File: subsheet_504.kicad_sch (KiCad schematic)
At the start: 36 parts, among them J502 Phono LEFT, J503 Phono RIGHT, U504 LF347N_mu, U508 LMC1992CCN_PHY

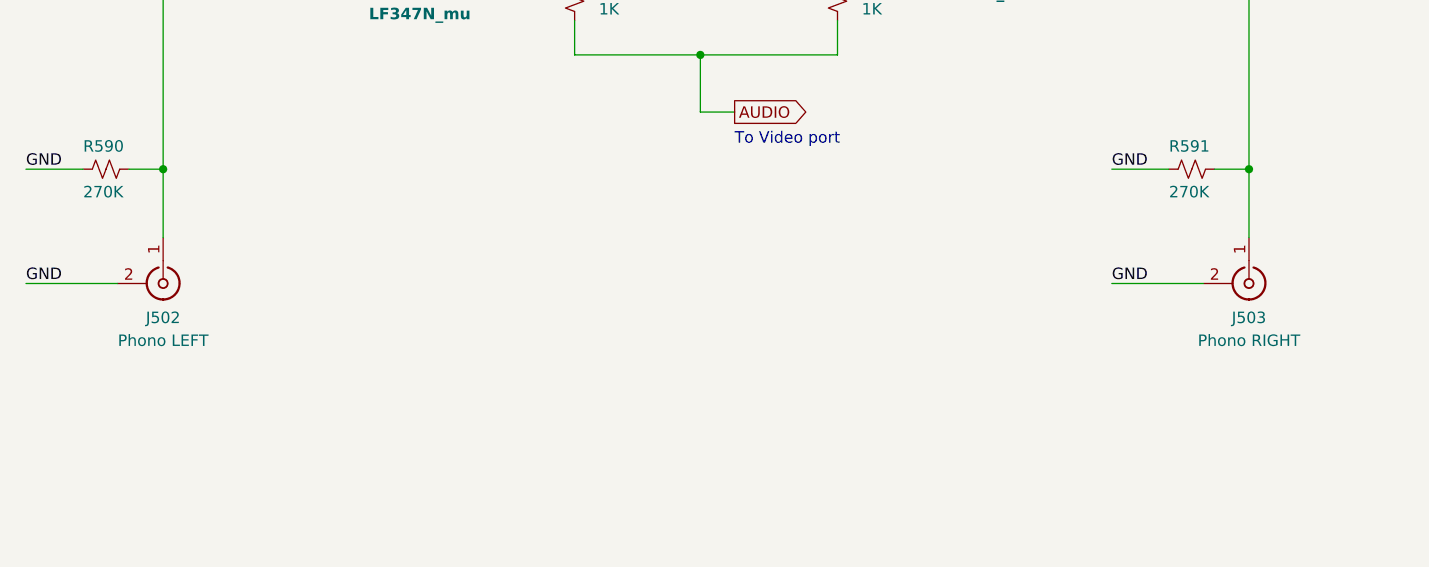
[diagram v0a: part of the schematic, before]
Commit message: pcb session 2023-01-21T22:41:51+01:00
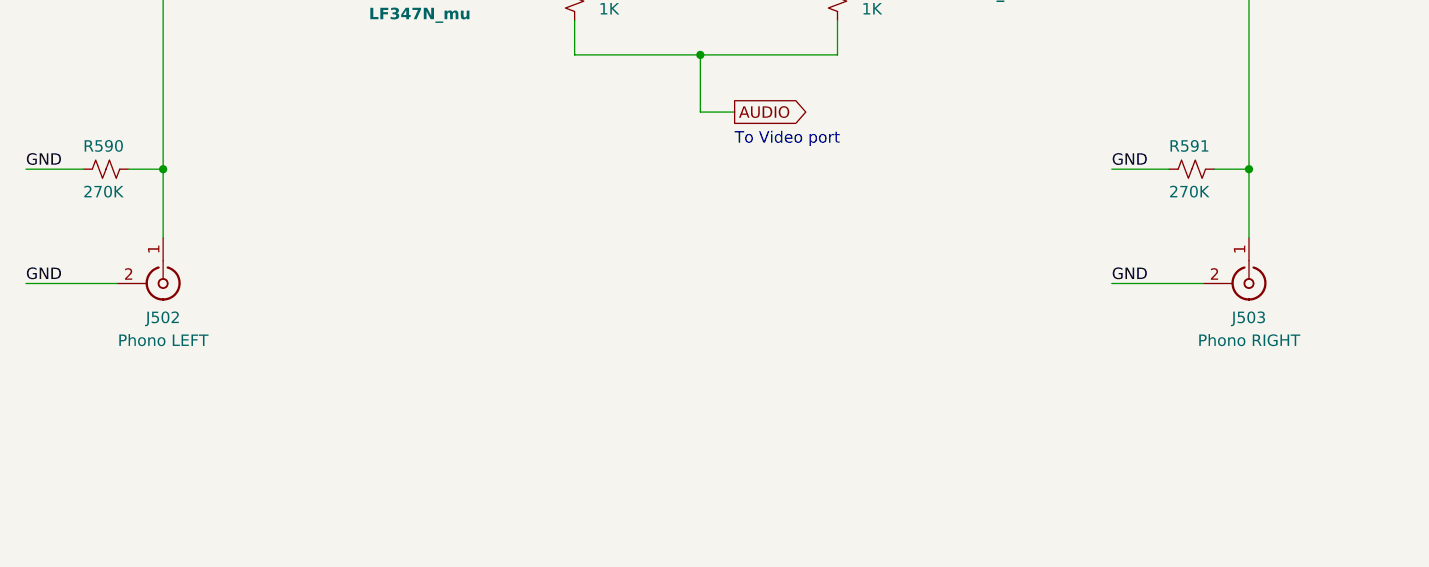
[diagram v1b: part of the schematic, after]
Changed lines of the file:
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@@
     (pin "9")
   )
-  (symbol (lib_id "Device:CP1") (at 88.9 59.69 0)
+  (symbol (lib_id "Device:CP1") (at 88.9 59.69 0) (unit 1)
     (in_bom yes) (on_board yes)
     (property "Reference" "CP535" (id 0) (at 90.17 57.15 0)
@@
     (pin "2")
   )
-  (symbol (lib_id "Device:R_Small_US") (at 76.2 59.69 0)
+  (symbol (lib_id "Device:R_Small_US") (at 76.2 59.69 0) (unit 1)
     (in_bom yes) (on_board yes)
     (property "Reference" "R530" (id 0) (at 77.47 58.42 0)
@@
     (pin "2")
   )
-  (symbol (lib_id "Device:C_Small") (at 101.6 59.69 0)
+  (symbol (lib_id "Device:C_Small") (at 101.6 59.69 0) (unit 1)
     (in_bom yes) (on_board yes)
     (property "Reference" "C536" (id 0) (at 102.87 57.15 0)
@@
     (pin "2")
   )
-  (symbol (lib_id "Device:CP1") (at 38.1 26.67 270)
+  (symbol (lib_id "Device:CP1") (at 38.1 26.67 270) (unit 1)
     (in_bom yes) (on_board yes)
     (property "Reference" "CP541" (id 0) (at 35.56 22.86 90)
@@
     (pin "2")
   )
-  (symbol (lib_id "Device:CP1") (at 38.1 39.37 270)
+  (symbol (lib_id "Device:CP1") (at 38.1 39.37 270) (unit 1)
     (in_bom yes) (on_board yes)
     (property "Reference" "CP546" (id 0) (at 35.56 35.56 90)
@@
     (pin "2")
   )
-  (symbol (lib_id "Device:CP1") (at 35.56 96.52 270)
+  (symbol (lib_id "Device:CP1") (at 35.56 96.52 270) (unit 1)
     (in_bom yes) (on_board yes)
     (property "Reference" "CP544" (id 0) (at 26.67 95.25 90)
@@
     (pin "2")
   )
-  (symbol (lib_id "Device:CP1") (at 172.72 93.98 90)
+  (symbol (lib_id "Device:CP1") (at 172.72 93.98 90) (unit 1)
     (in_bom yes) (on_board yes)
     (property "Reference" "CP547" (id 0) (at 170.18 92.71 90)
@@
     (pin "2")
   )
-  (symbol (lib_id "Device:R_Small_US") (at 88.9 25.4 0)
+  (symbol (lib_id "Device:R_Small_US") (at 88.9 25.4 0) (unit 1)
     (in_bom yes) (on_board yes)
     (property "Reference" "R525" (id 0) (at 90.17 24.13 0)
@@
     (pin "2")
   )
-  (symbol (lib_id "Device:R_Small_US") (at 78.74 33.02 90)
+  (symbol (lib_id "Device:R_Small_US") (at 78.74 33.02 90) (unit 1)
     (in_bom yes) (on_board yes)
     (property "Reference" "R531" (id 0) (at 81.28 30.48 90)
@@
     (pin "2")
   )
-  (symbol (lib_id "Device:R_Small_US") (at 97.79 41.91 180)
+  (symbol (lib_id "Device:R_Small_US") (at 97.79 41.91 180) (unit 1)
     (in_bom yes) (on_board yes)
     (property "Reference" "R539" (id 0) (at 104.14 40.64 0)
@@
     (pin "2")
   )
-  (symbol (lib_id "Device:C") (at 50.8 101.6 90)
+  (symbol (lib_id "Device:C") (at 50.8 101.6 90) (unit 1)
     (in_bom yes) (on_board yes)
     (property "Reference" "C528" (id 0) (at 49.53 102.87 90)
@@
     (pin "2")
   )
-  (symbol (lib_id "Device:C") (at 20.32 127 180)
+  (symbol (lib_id "Device:C") (at 20.32 127 180) (unit 1)
     (in_bom yes) (on_board yes)
     (property "Reference" "C531" (id 0) (at 27.94 125.73 0)
@@
     (pin "2")
   )
-  (symbol (lib_id "Device:C") (at 189.23 127 180)
+  (symbol (lib_id "Device:C") (at 189.23 127 180) (unit 1)
     (in_bom yes) (on_board yes)
     (property "Reference" "C534" (id 0) (at 185.42 125.73 0)
@@
     (pin "2")
   )
-  (symbol (lib_id "Device:C") (at 158.75 99.06 270)
+  (symbol (lib_id "Device:C") (at 158.75 99.06 270) (unit 1)
     (in_bom yes) (on_board yes)
     (property "Reference" "C538" (id 0) (at 160.02 100.33 90)
@@
     (pin "2")
   )
-  (symbol (lib_id "Device:C") (at 20.32 76.2 0)
+  (symbol (lib_id "Device:C") (at 20.32 76.2 0) (unit 1)
     (in_bom yes) (on_board yes)
     (property "Reference" "C524" (id 0) (at 20.955 73.66 0)
@@
     (pin "2")
   )
-  (symbol (lib_id "Device:R_Small_US") (at 44.45 139.7 180)
+  (symbol (lib_id "Device:R_Small_US") (at 44.45 139.7 180) (unit 1)
     (in_bom yes) (on_board yes)
     (property "Reference" "R520" (id 0) (at 40.64 138.43 0))
@@
     (pin "2")
   )
-  (symbol (lib_id "Device:CP1") (at 44.45 152.4 0)
+  (symbol (lib_id "Device:CP1") (at 44.45 152.4 0) (unit 1)
     (in_bom yes) (on_board yes)
     (property "Reference" "CP525" (id 0) (at 35.56 151.13 0)
@@
     (pin "2")
   )
-  (symbol (lib_id "Device:R_Small_US") (at 38.1 190.5 270)
+  (symbol (lib_id "Device:R_Small_US") (at 38.1 190.5 270) (unit 1)
     (in_bom yes) (on_board yes)
     (property "Reference" "R590" (id 0) (at 35.56 187.96 90)
@@
     (pin "2")
   )
-  (symbol (lib_id "Device:R_Small_US") (at 165.1 139.7 180)
+  (symbol (lib_id "Device:R_Small_US") (at 165.1 139.7 180) (unit 1)
     (in_bom yes) (on_board yes)
     (property "Reference" "R533" (id 0) (at 168.91 138.43 0))
@@
     (pin "2")
   )
-  (symbol (lib_id "Device:CP1") (at 165.1 152.4 0)
+  (symbol (lib_id "Device:CP1") (at 165.1 152.4 0) (unit 1)
     (in_bom yes) (on_board yes)
     (property "Reference" "CP537" (id 0) (at 167.64 151.13 0)
@@
     (pin "2")
   )
-  (symbol (lib_id "Device:R_Small_US") (at 158.75 190.5 270)
+  (symbol (lib_id "Device:R_Small_US") (at 158.75 190.5 270) (unit 1)
     (in_bom yes) (on_board yes)
     (property "Reference" "R591" (id 0) (at 156.21 187.96 90)
@@
     (pin "2")
   )
-  (symbol (lib_id "Device:CP1") (at 57.15 133.35 0)
+  (symbol (lib_id "Device:CP1") (at 57.15 133.35 0) (unit 1)
     (in_bom yes) (on_board yes)
     (property "Reference" "CP529" (id 0) (at 59.69 132.08 0)
@@
     (pin "2")
   )
-  (symbol (lib_id "Device:R_Small_US") (at 57.15 146.05 180)
+  (symbol (lib_id "Device:R_Small_US") (at 57.15 146.05 180) (unit 1)
     (in_bom yes) (on_board yes)
     (property "Reference" "R527" (id 0) (at 60.96 144.78 0))
@@
     (pin "2")
   )
-  (symbol (lib_id "Device:R_Small_US") (at 73.66 153.67 270)
+  (symbol (lib_id "Device:R_Small_US") (at 73.66 153.67 270) (unit 1)
     (in_bom yes) (on_board yes)
     (property "Reference" "R524" (id 0) (at 66.04 152.4 90)
@@
     (pin "2")
   )
-  (symbol (lib_id "Device:R_Small_US") (at 90.17 171.45 180)
+  (symbol (lib_id "Device:R_Small_US") (at 90.17 171.45 180) (unit 1)
     (in_bom yes) (on_board yes)
     (property "Reference" "R540" (id 0) (at 93.98 170.18 0))
@@
     (pin "2")
   )
-  (symbol (lib_id "Device:CP1") (at 152.4 133.35 0)
+  (symbol (lib_id "Device:CP1") (at 152.4 133.35 0) (unit 1)
     (in_bom yes) (on_board yes)
     (property "Reference" "CP543" (id 0) (at 154.94 132.08 0)
@@
     (pin "2")
   )
-  (symbol (lib_id "Device:R_Small_US") (at 152.4 146.05 180)
+  (symbol (lib_id "Device:R_Small_US") (at 152.4 146.05 180) (unit 1)
     (in_bom yes) (on_board yes)
     (property "Reference" "R538" (id 0) (at 156.21 144.78 0))
@@
     (pin "2")
   )
-  (symbol (lib_id "Device:R_Small_US") (at 135.89 153.67 90)
+  (symbol (lib_id "Device:R_Small_US") (at 135.89 153.67 90) (unit 1)
     (in_bom yes) (on_board yes)
     (property "Reference" "R537" (id 0) (at 133.35 152.4 90)
@@
     (pin "2")
   )
-  (symbol (lib_id "Device:R_Small_US") (at 119.38 171.45 180)
+  (symbol (lib_id "Device:R_Small_US") (at 119.38 171.45 180) (unit 1)
     (in_bom yes) (on_board yes)
     (property "Reference" "R541" (id 0) (at 123.19 170.18 0))
@@
     (pin "2")
   )
-  (symbol (lib_id "lf347:LF347N_mu") (at 73.66 166.37 0) (mirror x)
+  (symbol (lib_id "lf347:LF347N_mu") (at 73.66 166.37 0) (mirror x) (unit 1)
     (in_bom yes) (on_board yes)
     (property "Reference" "U504" (id 0) (at 67.31 171.45 0)
@@
       (effects (font (size 1.27 1.27)) (justify left top) hide)
     )
-    (pin "5")
-    (pin "6")
-    (pin "7")
-  )
-  (symbol (lib_id "lf347:LF347N_mu") (at 135.89 158.75 0) (mirror y)
+    (pin "1")
+    (pin "2")
+    (pin "3")
+  )
+  (symbol (lib_id "lf347:LF347N_mu") (at 135.89 158.75 0) (mirror y) (unit 1)
     (in_bom yes) (on_board yes)
     (property "Reference" "U504" (id 0) (at 135.89 167.64 0)
@@
       (effects (font (size 1.27 1.27)) (justify left top) hide)
     )
-    (pin "10")
-    (pin "8")
-    (pin "9")
-  )
-  (symbol (lib_id "Device:CP1") (at 154.94 81.28 90)
+    (pin "1")
+    (pin "2")
+    (pin "3")
+  )
+  (symbol (lib_id "Device:CP1") (at 154.94 81.28 90) (unit 1)
     (in_bom yes) (on_board yes)
     (property "Reference" "CP542" (id 0) (at 163.83 80.01 90)
@@
     (pin "2")
   )
-  (symbol (lib_id "Device:R_Small_US") (at 88.9 41.91 0)
+  (symbol (lib_id "Device:R_Small_US") (at 88.9 41.91 0) (unit 1)
     (in_bom yes) (on_board yes)
     (property "Reference" "R2701" (id 0) (at 90.17 40.64 0)
